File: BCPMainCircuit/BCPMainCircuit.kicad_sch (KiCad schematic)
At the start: 48 parts, among them Q1 IRLB8721PBF, SW1 Switch, U1 MCP9601T-E/MX, U2 Pico 2, U3 Logger, U4 GPS, U5 BNO055, U6 BME280, U7 MIC2940A-3.3WT, U8 MCP9601T-E/MX

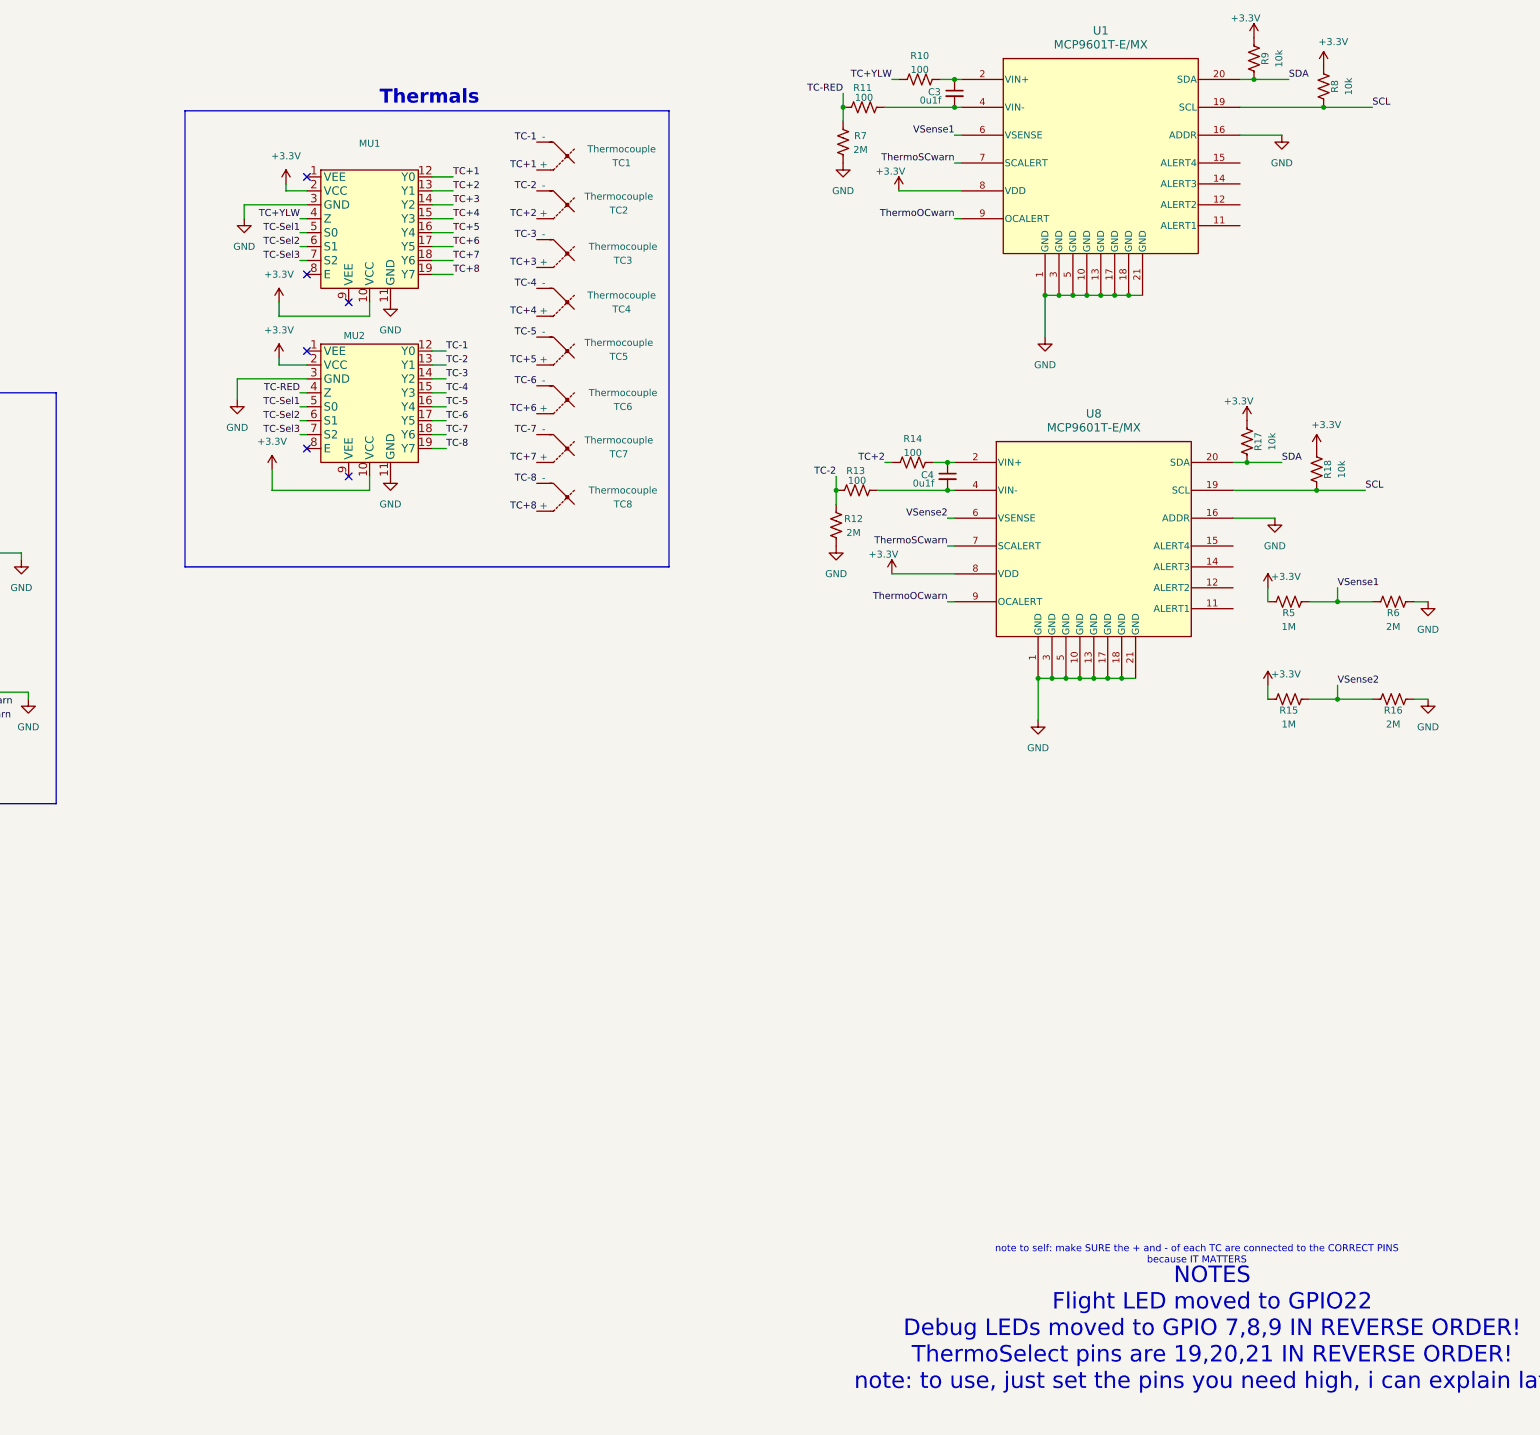
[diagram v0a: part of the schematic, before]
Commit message: minor changes n stuff
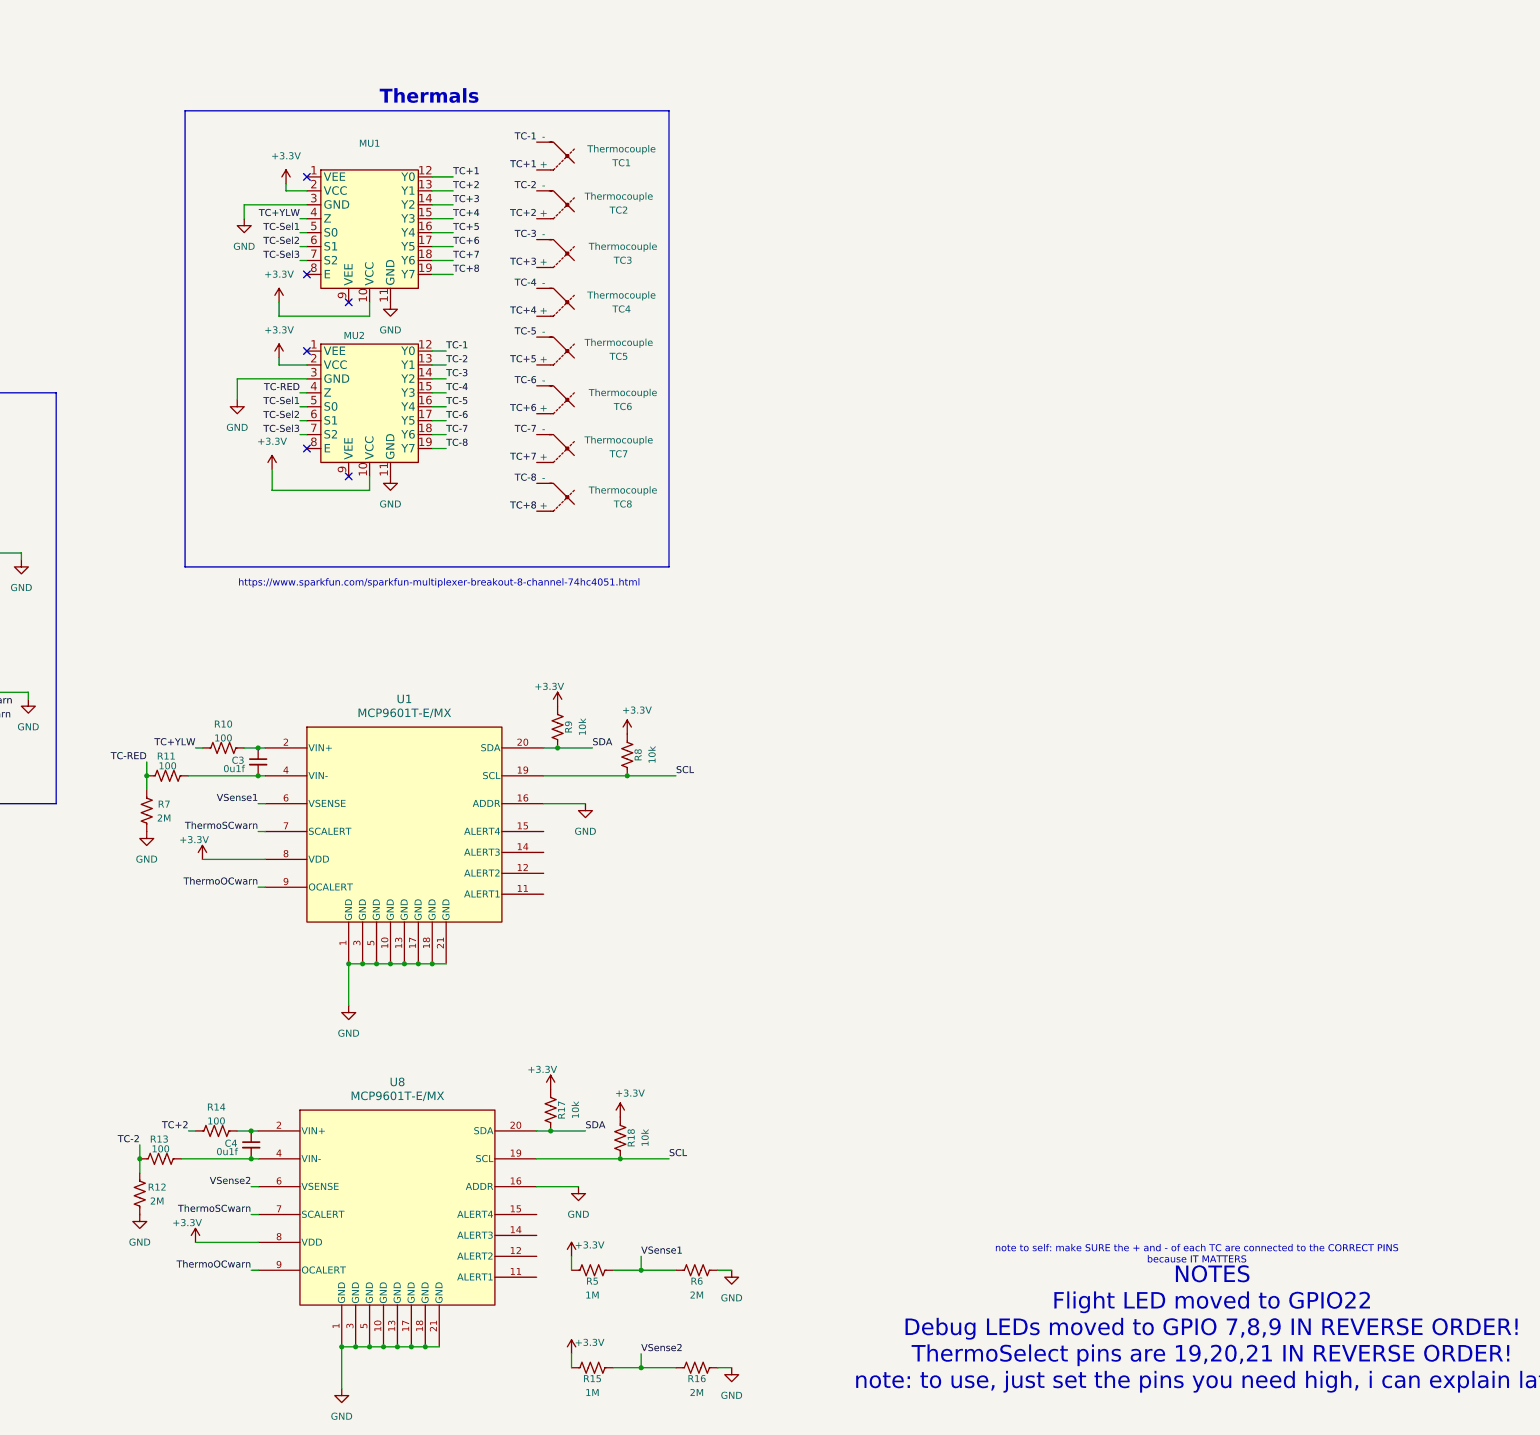
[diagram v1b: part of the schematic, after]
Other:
- note added: "https://www.sparkfun.com/sparkfun-multiplexer-breakout-8-channel-74hc4051.html"
- moved on the sheet: C3, C4, R10, R11, R12, R13, R14, R15, R16, R17, R18, R5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
